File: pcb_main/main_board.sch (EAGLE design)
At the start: 66 parts, among them IC7 LM1117IMPX-5.0, Q1 FDS5680, T1 BC847, U1 STM32F411RET6, X1 FH12-14S-0.5SH

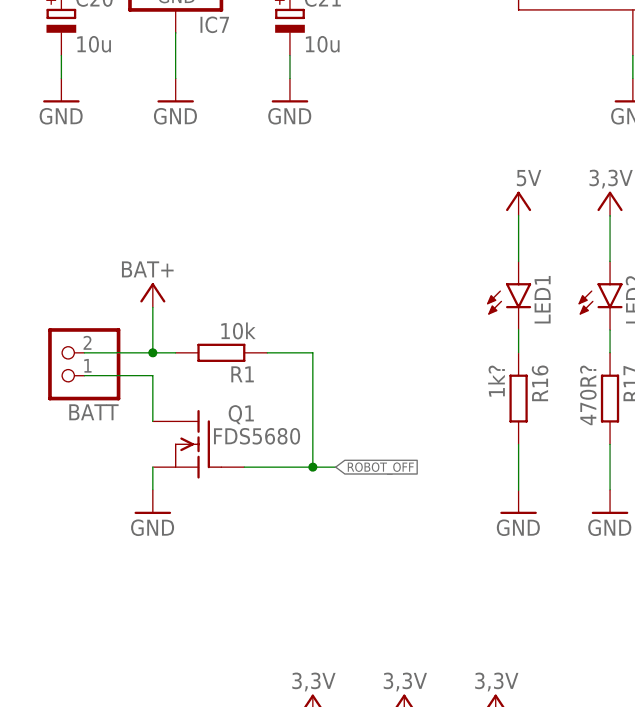
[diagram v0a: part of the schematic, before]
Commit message: corrected on
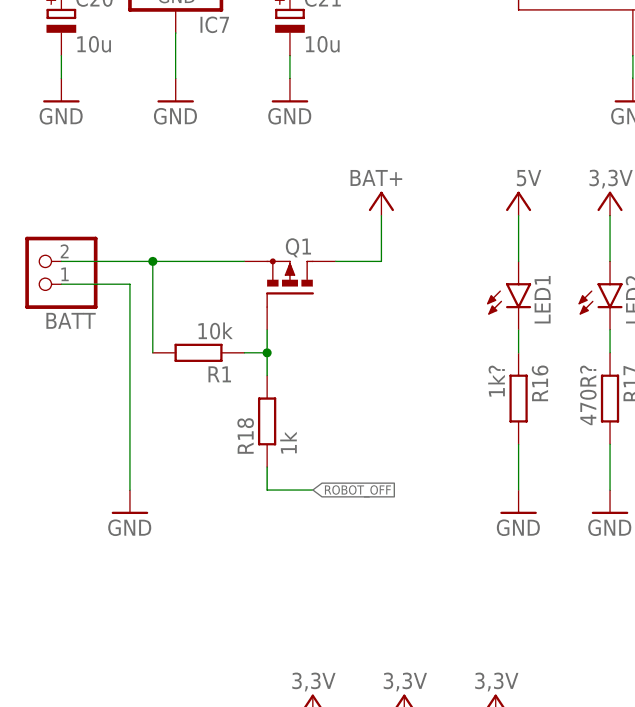
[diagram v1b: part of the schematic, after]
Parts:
- added R18: 1k, rcl:R-EU_R0603
- Q1: value FDS5680 -> (none); device transistor-fet:FDS5680 -> transistor-power:P-MOSFET-SO8
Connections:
- removed net BAT-: BATT.1, Q1.D
- new net BAT: BATT.2, Q1.S, R1.2
- new net N$8: Q1.G, R1.1, R18.2
- net BAT+: now also Q1.D; no longer BATT.2, R1.2
- net GND: now also BATT.1; no longer Q1.S
- net ROBOT_OFF: now also R18.1; no longer Q1.G, R1.1
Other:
- moved on the sheet: BATT, R1
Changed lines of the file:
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@@
 <part name="P+16" library="supply1" library_urn="urn:adsk.eagle:library:371" deviceset="VCC" device=""/>
 <part name="U$7" library="D24V10F3" deviceset="D24V10F3" device="-H" override_package3d_urn="urn:adsk.eagle:package:38702809/2" override_package_urn="urn:adsk.eagle:footprint:38702810/1"/>
-<part name="Q1" library="transistor-fet" library_urn="urn:adsk.eagle:library:396" deviceset="FDS5680" device="" package3d_urn="urn:adsk.eagle:package:28532/2"/>
 <part name="U$1" library="TOF_VL53L0X" deviceset="TOF_VL53L0X" device="" package3d_urn="urn:adsk.eagle:package:38702354/2"/>
 <part name="GND5" library="supply1" library_urn="urn:adsk.eagle:library:371" deviceset="GND" device=""/>
@@
 <part name="BATT" library="pinhead" library_urn="urn:adsk.eagle:library:325" deviceset="PINHD-1X2" device="" package3d_urn="urn:adsk.eagle:package:22435/2"/>
 <part name="GND2" library="supply1" library_urn="urn:adsk.eagle:library:371" deviceset="GND" device=""/>
-<part name="P+17" library="supply1" library_urn="urn:adsk.eagle:library:371" deviceset="VCC" device=""/>
 <part name="R1" library="rcl" library_urn="urn:adsk.eagle:library:334" deviceset="R-EU_" device="R0603" package3d_urn="urn:adsk.eagle:package:23555/3" value="10k"/>
 <part name="GND3" library="supply1" library_urn="urn:adsk.eagle:library:371" deviceset="GND" device=""/>
@@
 <part name="GND42" library="supply1" library_urn="urn:adsk.eagle:library:371" deviceset="GND" device=""/>
 <part name="P+37" library="supply1" library_urn="urn:adsk.eagle:library:371" deviceset="VCC" device=""/>
+<part name="Q1" library="transistor-power" library_urn="urn:adsk.eagle:library:400" deviceset="P-MOSFET-SO8" device="" package3d_urn="urn:adsk.eagle:package:20804/2"/>
+<part name="P+17" library="supply1" library_urn="urn:adsk.eagle:library:371" deviceset="VCC" device=""/>
+<part name="R18" library="rcl" library_urn="urn:adsk.eagle:library:334" deviceset="R-EU_" device="R0603" package3d_urn="urn:adsk.eagle:package:23555/3" value="1k"/>
 </parts>
 <sheets>
@@
 <wire x1="-55.88" y1="-96.52" x2="-55.88" y2="-43.18" width="0.1524" layer="90" style="shortdash"/>
 <wire x1="-55.88" y1="-43.18" x2="-160.02" y2="-43.18" width="0.1524" layer="90" style="shortdash"/>
-<wire x1="-281.94" y1="76.2" x2="-281.94" y2="-12.7" width="0.1524" layer="90" style="shortdash"/>
-<wire x1="-281.94" y1="-12.7" x2="-165.1" y2="-12.7" width="0.1524" layer="90" style="shortdash"/>
+<wire x1="-274.32" y1="76.2" x2="-274.32" y2="-12.7" width="0.1524" layer="90" style="shortdash"/>
+<wire x1="-274.32" y1="-12.7" x2="-165.1" y2="-12.7" width="0.1524" layer="90" style="shortdash"/>
 <wire x1="-165.1" y1="-12.7" x2="-165.1" y2="76.2" width="0.1524" layer="90" style="shortdash"/>
-<wire x1="-165.1" y1="76.2" x2="-281.94" y2="76.2" width="0.1524" layer="90" style="shortdash"/>
-<text x="-279.4" y="68.58" size="5.08" layer="90">Power</text>
+<wire x1="-165.1" y1="76.2" x2="-274.32" y2="76.2" width="0.1524" layer="90" style="shortdash"/>
+<text x="-271.78" y="68.58" size="5.08" layer="90">Power</text>
 <text x="121.92" y="68.58" size="5.08" layer="90">Motor driver</text>
 <text x="-157.48" y="-50.8" size="5.08" layer="90">Connectors</text>
@@
 <attribute name="VALUE" x="-200.66" y="43.18" size="1.778" layer="96"/>
 </instance>
-<instance part="Q1" gate="G$1" x="-251.46" y="0" smashed="yes" rot="MR0">
-<attribute name="VALUE" x="-240.03" y="0" size="1.778" layer="96" rot="MR0"/>
-<attribute name="NAME" x="-245.11" y="2.54" size="1.778" layer="95" rot="MR0"/>
-</instance>
 <instance part="U$1" gate="G$1" x="-144.78" y="38.1" smashed="yes">
 <attribute name="NAME" x="-144.78" y="35.56" size="1.778" layer="95"/>
@@
 </instance>
 <instance part="P+13" gate="VCC" x="-96.52" y="-10.16" smashed="yes"/>
-<instance part="BATT" gate="G$1" x="-266.7" y="10.16" smashed="yes" rot="R180">
-<attribute name="NAME" x="-260.35" y="4.445" size="1.778" layer="95" rot="R180"/>
-<attribute name="VALUE" x="-260.35" y="15.24" size="1.778" layer="96" rot="R180"/>
-</instance>
-<instance part="GND2" gate="1" x="-256.54" y="-7.62" smashed="yes">
-<attribute name="VALUE" x="-259.08" y="-10.16" size="1.778" layer="96"/>
-</instance>
-<instance part="P+17" gate="VCC" x="-256.54" y="17.78" smashed="yes"/>
-<instance part="R1" gate="G$1" x="-248.92" y="10.16" smashed="yes" rot="R180">
-<attribute name="NAME" x="-245.11" y="8.6614" size="1.778" layer="95" rot="R180"/>
-<attribute name="VALUE" x="-245.11" y="13.462" size="1.778" layer="96" rot="R180"/>
+<instance part="BATT" gate="G$1" x="-269.24" y="20.32" smashed="yes" rot="R180">
+<attribute name="NAME" x="-262.89" y="14.605" size="1.778" layer="95" rot="R180"/>
+<attribute name="VALUE" x="-262.89" y="25.4" size="1.778" layer="96" rot="R180"/>
+</instance>
+<instance part="GND2" gate="1" x="-259.08" y="-7.62" smashed="yes">
+<attribute name="VALUE" x="-261.62" y="-10.16" size="1.778" layer="96"/>
+</instance>
+<instance part="R1" gate="G$1" x="-251.46" y="10.16" smashed="yes" rot="R180">
+<attribute name="NAME" x="-247.65" y="8.6614" size="1.778" layer="95" rot="R180"/>
+<attribute name="VALUE" x="-247.65" y="13.462" size="1.778" layer="96" rot="R180"/>
 </instance>
 <instance part="GND3" gate="1" x="-203.2" y="38.1" smashed="yes">
@@
 </instance>
 <instance part="P+37" gate="VCC" x="-205.74" y="27.94" smashed="yes"/>
+<instance part="Q1" gate="G$1" x="-241.3" y="17.78" smashed="yes" rot="R90">
+<attribute name="NAME" x="-238.76" y="22.86" size="1.778" layer="95" rot="R180"/>
+<attribute name="VALUE" x="-241.3" y="22.86" size="1.778" layer="96" rot="R90"/>
+</instance>
+<instance part="P+17" gate="VCC" x="-231.14" y="27.94" smashed="yes"/>
+<instance part="R18" gate="G$1" x="-243.84" y="2.54" smashed="yes" rot="R90">
+<attribute name="NAME" x="-245.3386" y="-1.27" size="1.778" layer="95" rot="R90"/>
+<attribute name="VALUE" x="-240.538" y="-1.27" size="1.778" layer="96" rot="R90"/>
+</instance>
 </instances>
 <busses>
@@
 </segment>
 <segment>
-<pinref part="Q1" gate="G$1" pin="S"/>
-<pinref part="GND2" gate="1" pin="GND"/>
-<wire x1="-256.54" y1="-2.54" x2="-256.54" y2="-5.08" width="0.1524" layer="91"/>
-</segment>
-<segment>
 <pinref part="U$7" gate="G$1" pin="GND"/>
 <pinref part="GND3" gate="1" pin="GND"/>
@@
 <pinref part="GND42" gate="1" pin="GND"/>
 <wire x1="-205.74" y1="0" x2="-205.74" y2="-5.08" width="0.1524" layer="91"/>
+</segment>
+<segment>
+<pinref part="BATT" gate="G$1" pin="1"/>
+<wire x1="-259.08" y1="17.78" x2="-266.7" y2="17.78" width="0.1524" layer="91"/>
+<pinref part="GND2" gate="1" pin="GND"/>
+<wire x1="-259.08" y1="17.78" x2="-259.08" y2="-5.08" width="0.1524" layer="91"/>
 </segment>
 </net>
@@
 </segment>
 </net>
-<net name="BAT-" class="0">
-<segment>
-<pinref part="Q1" gate="G$1" pin="D"/>
-<wire x1="-256.54" y1="2.54" x2="-256.54" y2="7.62" width="0.1524" layer="91"/>
-<pinref part="BATT" gate="G$1" pin="1"/>
-<wire x1="-256.54" y1="7.62" x2="-264.16" y2="7.62" width="0.1524" layer="91"/>
-</segment>
-</net>
 <net name="BAT+" class="0">
-<segment>
-<pinref part="P+17" gate="VCC" pin="VCC"/>
-<wire x1="-256.54" y1="15.24" x2="-256.54" y2="10.16" width="0.1524" layer="91"/>
-<pinref part="BATT" gate="G$1" pin="2"/>
-<wire x1="-256.54" y1="10.16" x2="-264.16" y2="10.16" width="0.1524" layer="91"/>
-<label x="-254" y="20.32" size="1.778" layer="95" rot="R180"/>
-<pinref part="R1" gate="G$1" pin="2"/>
-<wire x1="-254" y1="10.16" x2="-256.54" y2="10.16" width="0.1524" layer="91"/>
-<junction x="-256.54" y="10.16"/>
-</segment>
 <segment>
 <pinref part="U$7" gate="G$1" pin="VIN"/>
@@
 <junction x="-266.7" y="53.34"/>
 </segment>
+<segment>
+<pinref part="P+17" gate="VCC" pin="VCC"/>
+<wire x1="-231.14" y1="25.4" x2="-231.14" y2="20.32" width="0.1524" layer="91"/>
+<label x="-228.6" y="30.48" size="1.778" layer="95" rot="R180"/>
+<pinref part="Q1" gate="G$1" pin="D"/>
+<wire x1="-236.22" y1="20.32" x2="-231.14" y2="20.32" width="0.1524" layer="91"/>
+</segment>
 </net>
 <net name="ROBOT_OFF" class="0">
 <segment>
-<pinref part="R1" gate="G$1" pin="1"/>
-<wire x1="-243.84" y1="10.16" x2="-238.76" y2="10.16" width="0.1524" layer="91"/>
-<pinref part="Q1" gate="G$1" pin="G"/>
-<wire x1="-238.76" y1="10.16" x2="-238.76" y2="-2.54" width="0.1524" layer="91"/>
-<wire x1="-238.76" y1="-2.54" x2="-246.38" y2="-2.54" width="0.1524" layer="91"/>
-<wire x1="-238.76" y1="-2.54" x2="-236.22" y2="-2.54" width="0.1524" layer="91"/>
-<junction x="-238.76" y="-2.54"/>
-<label x="-236.22" y="-2.54" size="1.016" layer="95" xref="yes"/>
+<label x="-238.76" y="-5.08" size="1.016" layer="95" xref="yes"/>
+<wire x1="-243.84" y1="-2.54" x2="-243.84" y2="-5.08" width="0.1524" layer="91"/>
+<pinref part="R18" gate="G$1" pin="1"/>
+<wire x1="-243.84" y1="-5.08" x2="-238.76" y2="-5.08" width="0.1524" layer="91"/>
 </segment>
 <segment>
@@
 </segment>
 </net>
+<net name="BAT" class="0">
+<segment>
+<pinref part="BATT" gate="G$1" pin="2"/>
+<wire x1="-246.38" y1="20.32" x2="-256.54" y2="20.32" width="0.1524" layer="91"/>
+<pinref part="Q1" gate="G$1" pin="S"/>
+<pinref part="R1" gate="G$1" pin="2"/>
+<wire x1="-256.54" y1="20.32" x2="-266.7" y2="20.32" width="0.1524" layer="91"/>
+<wire x1="-256.54" y1="10.16" x2="-256.54" y2="20.32" width="0.1524" layer="91"/>
+<junction x="-256.54" y="20.32"/>
+</segment>
+</net>
+<net name="N$8" class="0">
+<segment>
+<pinref part="R1" gate="G$1" pin="1"/>
+<wire x1="-246.38" y1="10.16" x2="-243.84" y2="10.16" width="0.1524" layer="91"/>
+<pinref part="Q1" gate="G$1" pin="G"/>
+<wire x1="-243.84" y1="10.16" x2="-243.84" y2="12.7" width="0.1524" layer="91"/>
+<pinref part="R18" gate="G$1" pin="2"/>
+<wire x1="-243.84" y1="7.62" x2="-243.84" y2="10.16" width="0.1524" layer="91"/>
+<junction x="-243.84" y="10.16"/>
+</segment>
+</net>
